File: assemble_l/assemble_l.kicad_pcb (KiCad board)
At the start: 2 copper layers, 128.5 x 92.1 mm, 45 parts, among them J1 Conn_01x02_Pin, SW1 SW_Push, SW10 SW_Push, SW11 SW_Push, SW12 SW_Push, SW13 SW_Push, SW14 SW_Push, SW15 SW_Push, SW16 SW_Push, SW17 SW_Push, SW18 SW_Push, SW19 SW_Push, SW2 SW_Push, SW20 SW_Push, SW21 SW_Push, SW22 SW_Push, SW3 SW_Push, SW4 SW_Push, SW5 SW_Push, SW6 SW_Push, SW7 SW_Push, SW8 SW_Push, SW9 SW_Push, U1 Micon_BLEMicroPro

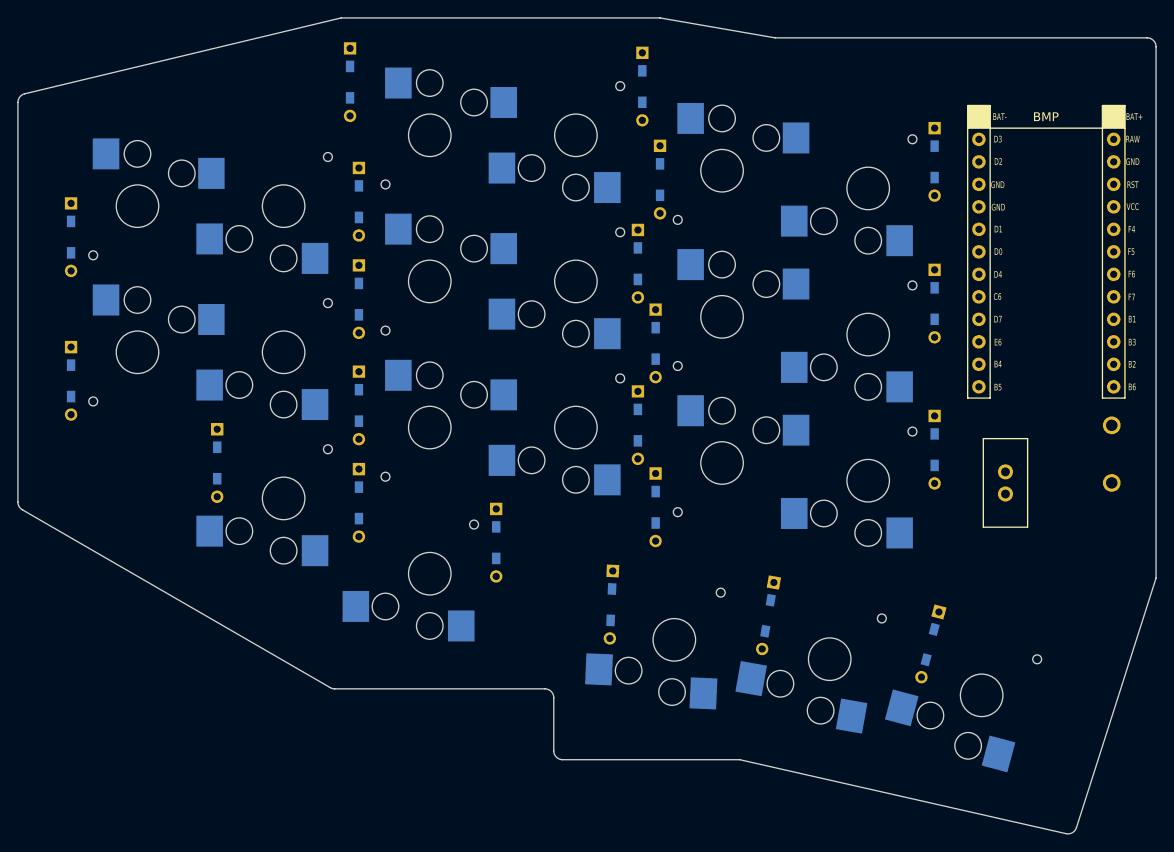
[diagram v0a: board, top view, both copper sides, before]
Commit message: fix: re-change layout
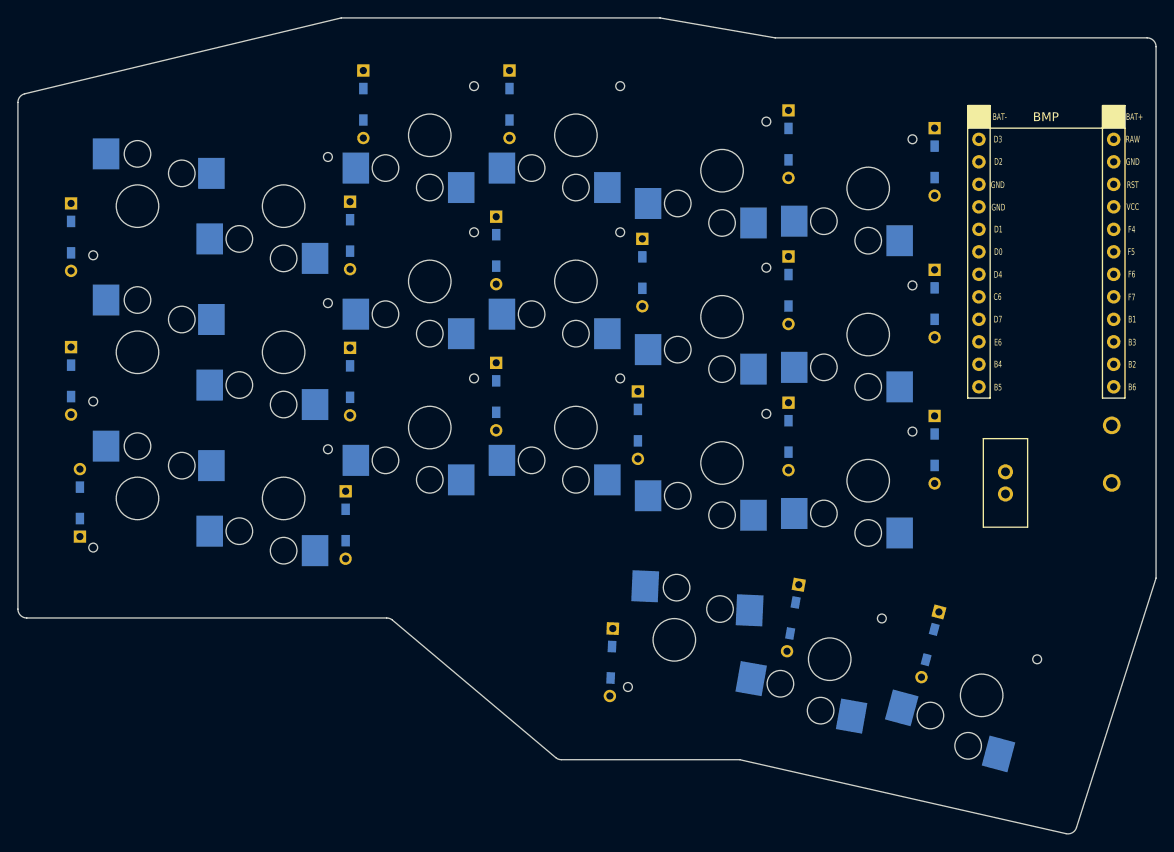
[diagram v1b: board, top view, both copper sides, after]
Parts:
- moved D3 46.3 mm to (61.5, 81.0), turned to 90 degrees
- moved SW3 36.9 mm to (68.0, 80.5), turned to 180 degrees
- moved D8 19.6 mm to (108.5, 69.0)
- moved D4 19.2 mm to (92.0, 50.8)
- moved SW9 18.6 mm to (84.5, 80.5)
- moved D5 17.6 mm to (92.0, 67.3)
- moved D9 17.1 mm to (91.5, 83.5)
- moved D16 17.0 mm to (141.5, 73.5)
- moved SW4 16.5 mm to (84.5, 47.5)
- moved SW5 16.5 mm to (84.5, 64.0)
- moved D7 16.4 mm to (108.5, 52.5)
- moved D15 16.2 mm to (141.5, 57.0)
- moved D10 15.1 mm to (110.0, 36.0)
- moved D14 15.0 mm to (141.5, 40.5)
- moved D13 6.50 mm to (121.5, 99.0)
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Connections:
- D3 pad 1: Row0 -> Row2
- D4 pad 1: Row1 -> Row0
- D5 pad 1: Row2 -> Row1
- D6 pad 1: Row0 -> Row2
- D7 pad 1: Row1 -> Row0
- D8 pad 1: Row2 -> Row1
- D9 pad 1: Row3 -> Row2
- SW3 pad 1: Col1 -> Col0
- SW6 pad 1: Col2 -> Col1
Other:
- outline, holes or cut-outs redrawn
